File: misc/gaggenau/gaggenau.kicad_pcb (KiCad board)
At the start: 2 copper layers, 51.1 x 104.5 mm, 51 parts, among them IC1 ESP32-C6-WROOM-1-N8, J1 Mains, J10 VentX, J2 Vent, J3 Conn_01x08_Socket, J4 Light, J7 ?, J8 ? Klemmen, Q10 Q_PMOS, Q11 Q_PMOS, Q12 Q_PMOS, Q13 Q_PMOS, Q14 Q_NMOS, Q2 BTB16-600BW, Q9 Q_NMOS, U1 PC-817, U4 KMOC302S, U5 CPC1965G

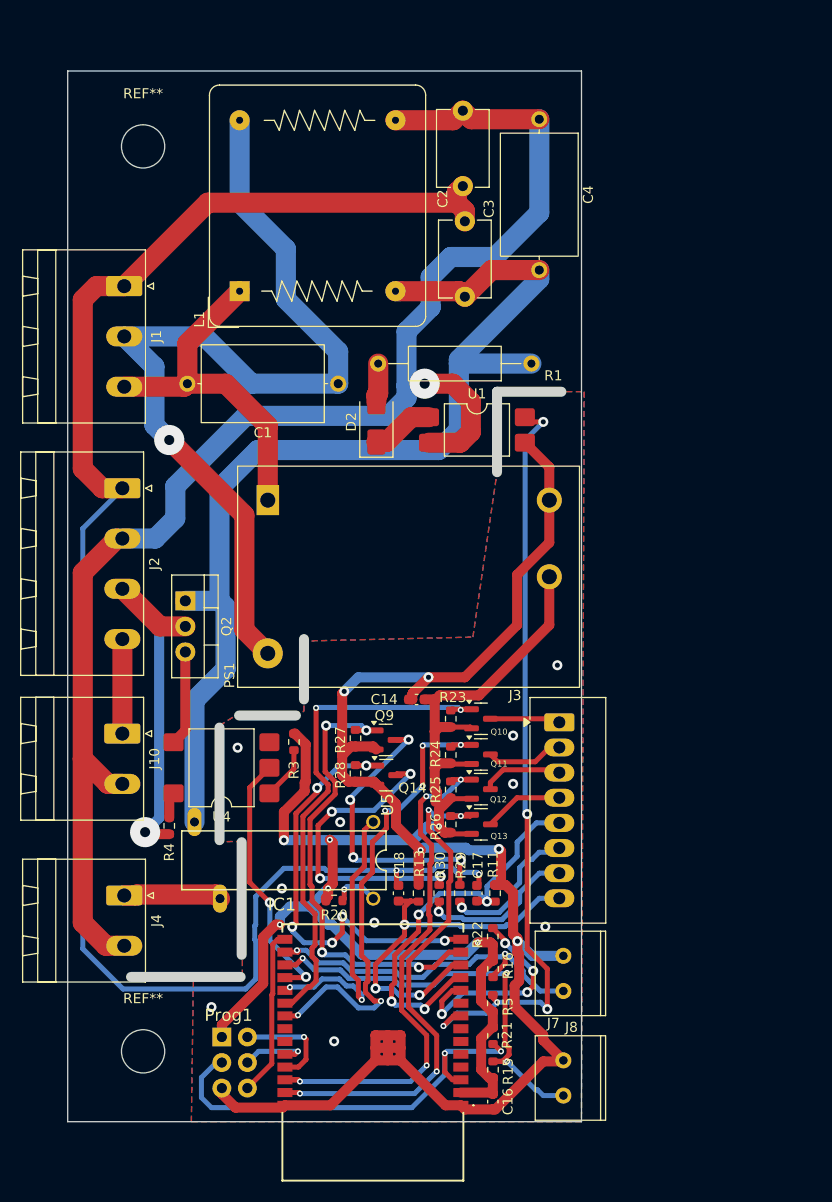
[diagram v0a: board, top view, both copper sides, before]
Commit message: Gaggenau replacement v2
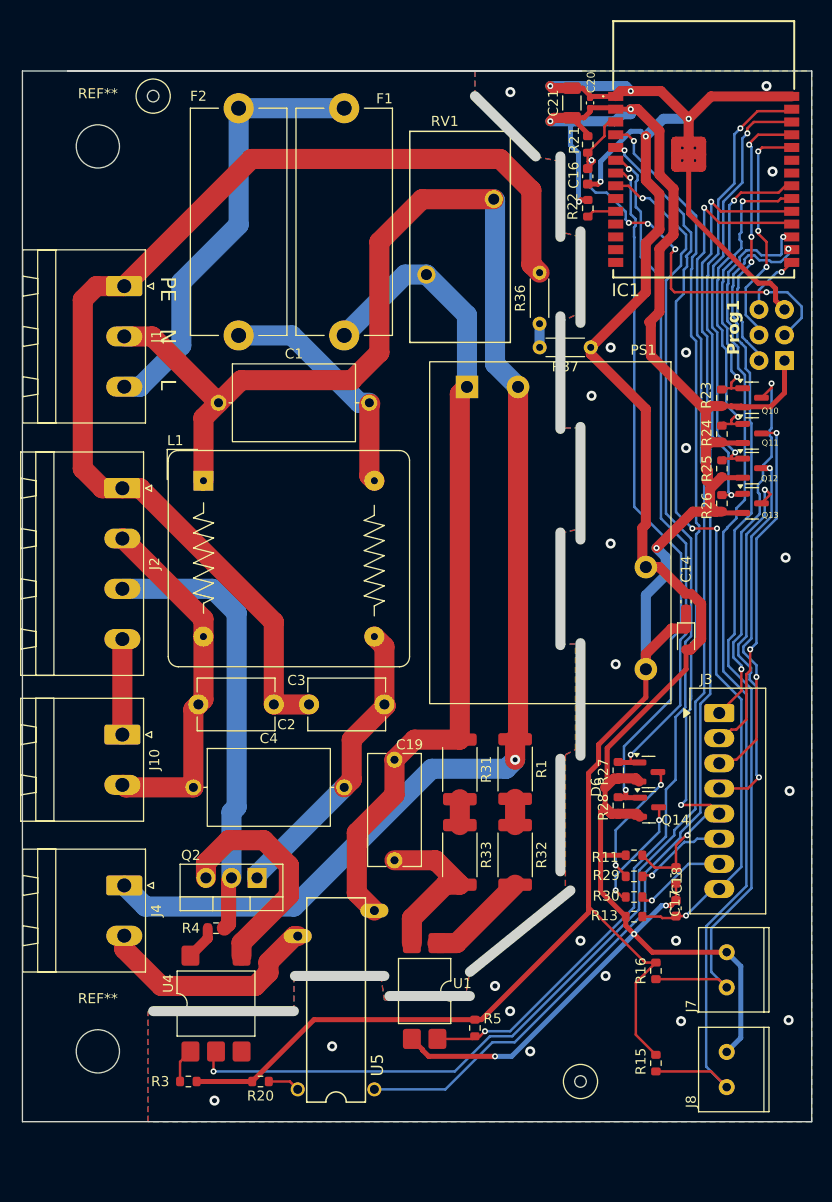
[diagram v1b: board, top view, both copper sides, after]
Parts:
- removed D2: S1A-13F, Diode_SMD:D_SMA
- added C19: 22nF 400V X2, Capacitor_THT:C_Rect_L11.0mm_W5.1mm_P10.00mm_MKT, F.Cu at (41.0, 81.0)
- added C20: 100nF, Capacitor_SMD:C_0402_1005Metric, F.Cu at (60.5, 15.7)
- added C21: 22µF, Capacitor_SMD:C_1206_3216Metric, F.Cu at (58.6, 15.7)
- added D6: ESDA041, Diode_SMD:D_SOD-323, F.Cu at (70.0, 69.0)
- added F1: FuseHolder, Fuse:Fuseholder_Cylinder-5x20mm_Stelvio-Kontek_PTF78_Horizontal_Open, F.Cu at (36.0, 38.8)
- added F2: FuseHolder, Fuse:Fuseholder_Cylinder-5x20mm_Stelvio-Kontek_PTF78_Horizontal_Open, F.Cu at (25.5, 38.8)
- added R31: 470 100V, Resistor_SMD:R_2512_6332Metric, F.Cu at (47.5, 82.0)
- added R32: 2k2, Resistor_SMD:R_2512_6332Metric, F.Cu at (53.0, 90.5)
- added R33: 470 100V, Resistor_SMD:R_2512_6332Metric, F.Cu at (47.5, 90.5)
- added R36: 1M, Resistor_THT:R_Axial_DIN0204_L3.6mm_D1.6mm_P5.08mm_Horizontal, F.Cu at (55.4, 37.6)
- added R37: 1M, Resistor_THT:R_Axial_DIN0204_L3.6mm_D1.6mm_P5.08mm_Horizontal, F.Cu at (60.5, 40.0)
- added REF**: TestPoint_Plated_Hole_D2.0mm, TestPoint:TestPoint_Plated_Hole_D2.0mm, F.Cu at (59.5, 113.0)
- added REF**: TestPoint_Plated_Hole_D2.0mm, TestPoint:TestPoint_Plated_Hole_D2.0mm, F.Cu at (17.0, 15.0)
- added RV1: Varistor230V, localstuff:Varistor_Disc_D21mm_W10mm_P7.5mm, F.Cu at (44.2, 32.8)
- C16: value 10µF -> 10nF
- PS1: value RAC01-3.3 -> Apos03; footprint localstuff:RAC01-3.3 -> localstuff:Hiecube AP05-Zero
- R1: value 22k -> 2k2; footprint Resistor_THT:R_Axial_DIN0309_L9.0mm_D3.2mm_P15.24mm_Horizontal -> Resistor_SMD:R_2512_6332Metric
- U1: value PC-817 -> PC814
- moved IC1 95.7 mm to (71.8, 20.3), turned to 0 degrees
- moved C16 92.5 mm to (60.2, 23.0), turned to -90 degrees
- moved Prog1 89.9 mm to (78.5, 38.8), turned to 90 degrees
- moved R21 89.1 mm to (60.2, 19.8)
- moved C4 74.8 mm to (21.0, 83.8), turned to 0 degrees
- moved R22 73.0 mm to (60.2, 26.2)
- moved C2 64.6 mm to (21.5, 75.5), turned to 0 degrees
- moved U1 56.0 mm to (44.0, 104.0), turned to -90 degrees
- moved C3 50.5 mm to (32.5, 75.5), turned to 0 degrees
- moved R24 41.8 mm to (73.6, 48.6)
- moved Q10 41.8 mm to (76.6, 45.0)
- moved Q11 41.8 mm to (76.6, 48.5)
- moved Q12 41.8 mm to (76.6, 52.0)
- moved Q13 41.8 mm to (76.6, 55.5)
- moved R23 41.8 mm to (73.6, 45.0)
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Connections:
- C1 pad 1: Net-(J1-Pin_2) -> /N
- C1 pad 2: Net-(J1-Pin_3) -> Net-(C1-Pad2)
- C16 pad 1: GND -> /EN
- C16 pad 2: VCC -> GND
- C17 pad 2: Earth_Protective -> GND
- C18 pad 2: Earth_Protective -> GND
- C2 pad 1: /N -> /Nx
- C3 pad 2: /L -> /Lx
- C4 pad 1: /N -> /Nx
- C4 pad 2: /L -> /Lx
- IC1 pad 11: /Btn5 -> unconnected-(IC1-IO10-Pad11)
- IC1 pad 12: /Btn6 -> unconnected-(IC1-IO11-Pad12)
- IC1 pad 13: /Btn7 -> unconnected-(IC1-IO12-Pad13)
- IC1 pad 14: /Btn8 -> unconnected-(IC1-IO13-Pad14)
- IC1 pad 4: unconnected-(IC1-IO4-Pad4) -> /Btn5
- IC1 pad 5: unconnected-(IC1-IO5-Pad5) -> /Btn6
- IC1 pad 6: unconnected-(IC1-IO6-Pad6) -> /Btn7
- IC1 pad 7: unconnected-(IC1-IO7-Pad7) -> /Btn8
- J1 pad 2: Net-(J1-Pin_2) -> /N
- J1 pad 3: Net-(J1-Pin_3) -> /L
- J10 pad 2: /N -> /Nx
- J2 pad 2: /N -> /Nx
- J4 pad 1: /Llight -> /N
- J4 pad 2: /N -> /Llight
- L1 pad 1: Net-(J1-Pin_3) -> /N
- L1 pad 2: /L -> /Nx
- L1 pad 3: Net-(J1-Pin_2) -> Net-(C1-Pad2)
- L1 pad 4: /N -> /Lx
- PS1 pad 1: Net-(J1-Pin_3) -> /Lf
- PS1 pad 2: Net-(J1-Pin_2) -> /N
- PS1 pad 3: GND -> VCC
- PS1 pad 4: VCC -> GND
- Q2 pad 1: /L -> /Lx
- R1 pad 1: /L -> /N
- R22 pad 1: Net-(IC1-IO8) -> VCC
- R22 pad 2: VCC -> Net-(IC1-IO8)
- U1 pad 2: /N -> Net-(C19-Pad2)
- U5 pad 8: /L -> /Lf
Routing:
- net /OVent: track 26.1 -> 133.5 mm
- net Net-(J1-Pin_2): track 90.9 -> 0.00 mm, vias 1 -> 0
- net /Olight: track 27.9 -> 116.7 mm, vias 2 -> 1
- net /Lf: track 0.00 -> 83.5 mm
- net GND: track 163.7 -> 247.1 mm, vias 15 -> 28
- net VCC: track 143.3 -> 219.2 mm, vias 6 -> 4
- net /L: track 106.9 -> 43.8 mm
- net /PB2: track 42.6 -> 103.2 mm, vias 3 -> 1
- net /PB1: track 34.8 -> 91.3 mm, vias 2 -> 1
- net Earth_Protective: track 168.0 -> 114.1 mm, vias 2 -> 0
- net /Btn6: track 38.7 -> 91.9 mm, vias 3 -> 4
- net /Btn5: track 40.2 -> 87.9 mm, vias 4 -> 3
- net /Nx: track 0.00 -> 35.7 mm
- net Net-(J1-Pin_3): track 34.9 -> 0.00 mm
- net /Kblau: track 6.50 -> 37.7 mm, vias 0 -> 2
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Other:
- board size 51.1 x 104.5 mm -> 78.5 x 104.5 mm
- board text added: "Dr"
- board text added: "Drossel"
- board text added: "L"
- board text added: "Licht"
- board text added: "Lüfter"
- board text added: "MoaT Ersatz + Update für Gaggenau 00263145 V 2.0"
- board text added: "N"
- board text added: "Netz"
- board text added: "PE"
